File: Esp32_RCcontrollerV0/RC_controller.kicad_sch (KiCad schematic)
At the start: 15 parts, among them J1 Conn_01x03_Pin, J2 Conn_01x03_Pin, J3 Conn_01x02_Socket, J4 Conn_01x02_Socket, J5 5V_Signal, J6 5V_Signal, J7 INPUT POWER (12 - 24V), U1 XL1509-5.0, U2 NODEMCU-32S, U4 BOB-12009, U5 BOB-12009

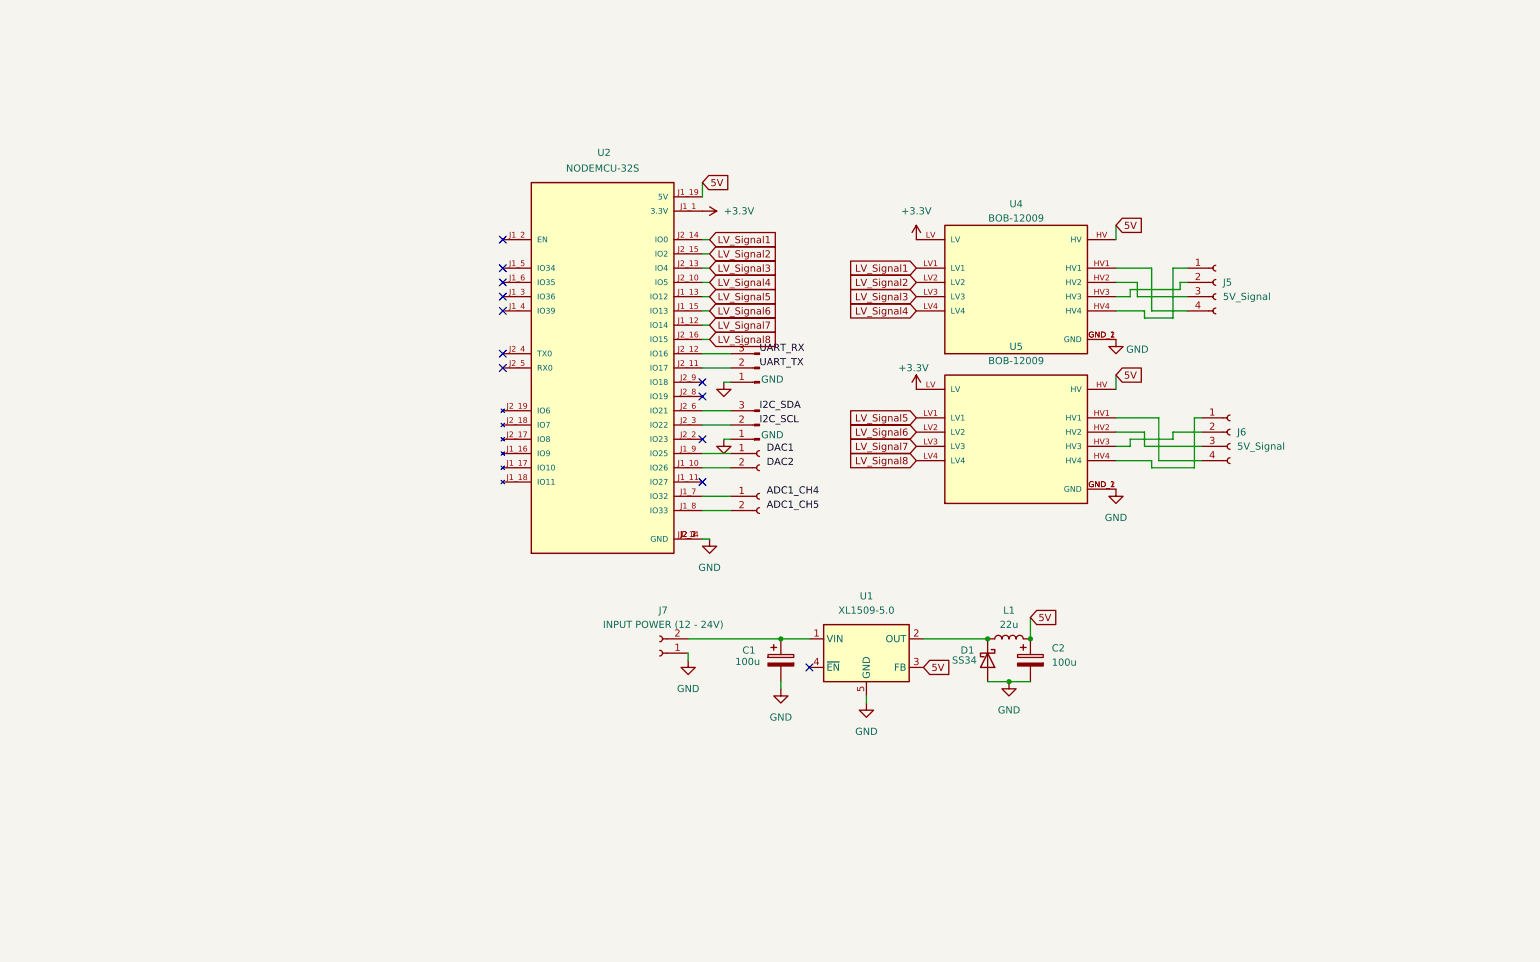
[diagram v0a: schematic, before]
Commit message: Core updates
Rework the board , Added Doc
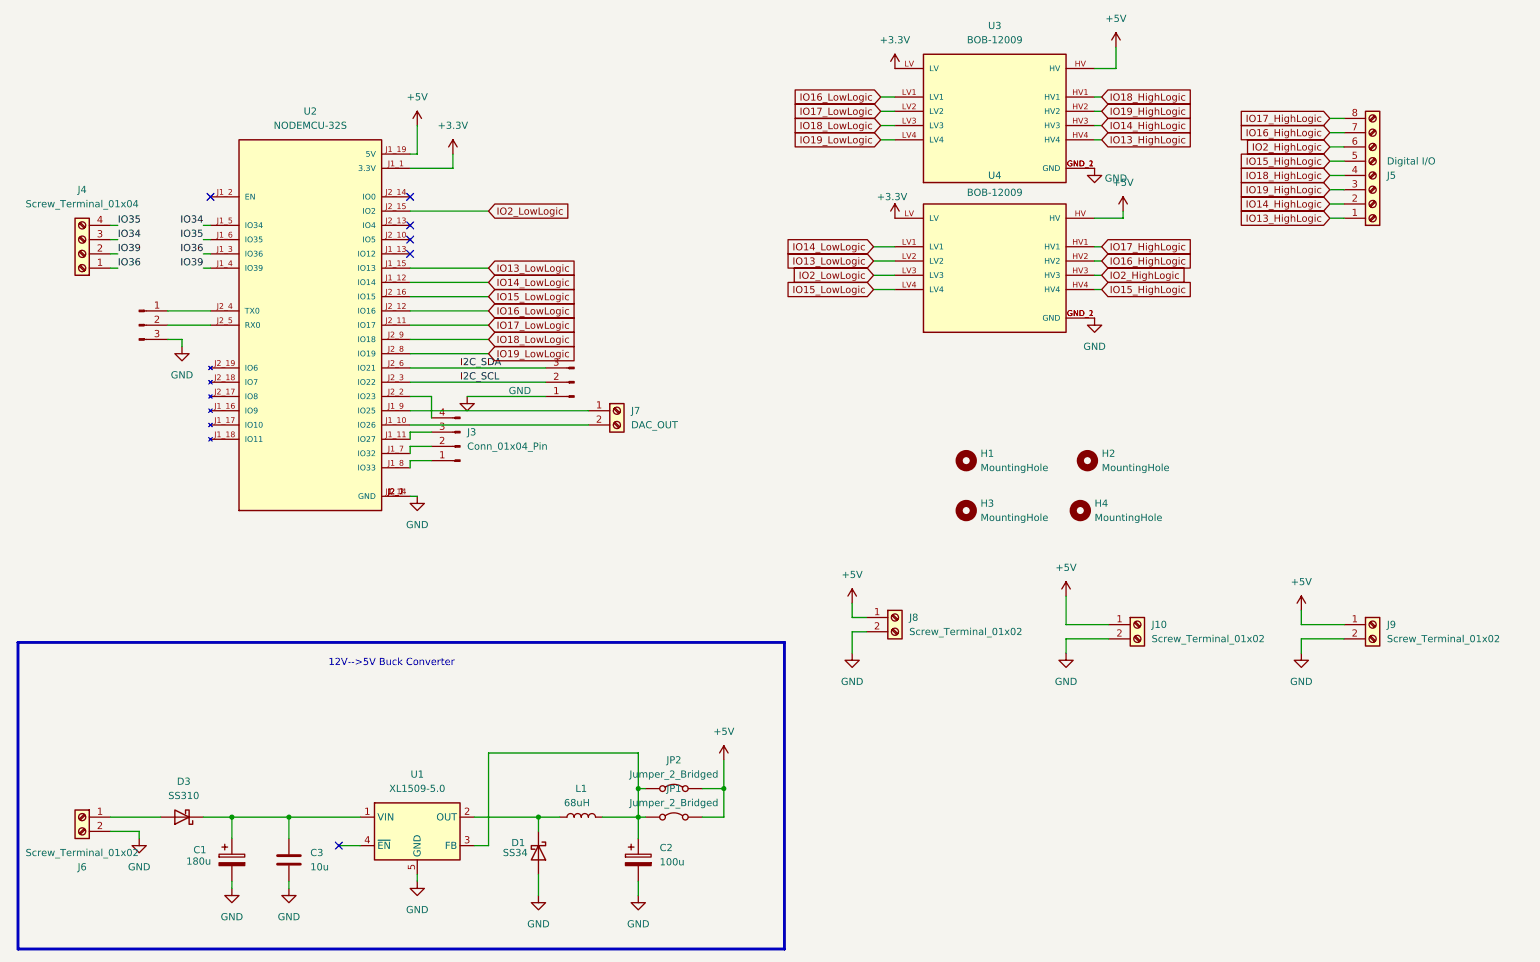
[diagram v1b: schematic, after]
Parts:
- removed J3, J4: Conn_01x02_Socket, TerminalBlock_Phoenix:TerminalBlock_Phoenix_PT-1,5-2-3.5-H_1x02_P3.50mm_Horizontal, symbol Connector:Conn_01x02_Socket
- removed J5, J6: 5V_Signal, TerminalBlock_Phoenix:TerminalBlock_Phoenix_PT-1,5-4-3.5-H_1x04_P3.50mm_Horizontal, symbol Connector:Conn_01x04_Socket
- removed J7: INPUT POWER (12 - 24V), TerminalBlock_Phoenix:TerminalBlock_Phoenix_MKDS-1,5-2-5.08_1x02_P5.08mm_Horizontal, symbol Connector:Conn_01x02_Socket
- removed U2: NODEMCU-32S, NODEMCU-32S:MODULE_NODEMCU-32S, symbol NODEMCU-32S:NODEMCU-32S
- removed U4, U5: BOB-12009, BOB-12009:CONV_BOB-12009, symbol BOB-12009:BOB-12009
- added C3: 10u, Capacitor_SMD:C_1206_3216Metric_Pad1.33x1.80mm_HandSolder, symbol Device:C
- added D3: SS310, Diode_SMD:D_SMA, symbol Diode:SS310
- added H1, H2, H3, H4: MountingHole, MountingHole:MountingHole_3.2mm_M3, symbol Mechanical:MountingHole
- added J10, J6, J8, J9: Screw_Terminal_01x02, TerminalBlock_Phoenix:TerminalBlock_Phoenix_PT-1,5-2-3.5-H_1x02_P3.50mm_Horizontal, symbol Connector:Screw_Terminal_01x02
- added J3: Conn_01x04_Pin, Connector_PinHeader_2.54mm:PinHeader_1x04_P2.54mm_Vertical, symbol Connector:Conn_01x04_Pin
- added J4: Screw_Terminal_01x04, TerminalBlock_Phoenix:TerminalBlock_Phoenix_PT-1,5-4-3.5-H_1x04_P3.50mm_Horizontal, symbol Connector:Screw_Terminal_01x04
- added J5: Digital I/O, TerminalBlock_Phoenix:TerminalBlock_Phoenix_PT-1,5-8-3.5-H_1x08_P3.50mm_Horizontal, symbol Connector:Screw_Terminal_01x08
- added J7: DAC_OUT, TerminalBlock_Phoenix:TerminalBlock_Phoenix_PT-1,5-2-3.5-H_1x02_P3.50mm_Horizontal, symbol Connector:Screw_Terminal_01x02
- added JP1, JP2: Jumper_2_Bridged, Connector_PinHeader_2.54mm:PinHeader_1x02_P2.54mm_Vertical, symbol Jumper:Jumper_2_Bridged
- added U2: NODEMCU-32S, LibMain:MODULE_NODEMCU-32S, symbol LibMain:NODEMCU-32S
- added U3, U4: BOB-12009, LibMain:CONV_BOB-12009, symbol LibMain:BOB-12009
- C1: value 100u -> 180u; footprint Capacitor_SMD:CP_Elec_10x10 -> Capacitor_THT:CP_Radial_D7.5mm_P2.50mm
- C2: footprint Capacitor_SMD:CP_Elec_6.3x5.8 -> Capacitor_THT:CP_Radial_D7.5mm_P2.50mm
- J1, J2: footprint Connector_JST:JST_EH_B3B-EH-A_1x03_P2.50mm_Vertical -> Connector_PinHeader_2.54mm:PinHeader_1x03_P2.54mm_Vertical
- L1: value 22u -> 68uH; footprint Inductor_SMD:L_APV_ANR5020 -> EasyEDA:IND-SMD_L7.1-W6.6_H5.0
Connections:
- net +3.3V: now also U2.J1_1 (3.3V), U3.LV, U4.LV
- net GND: now also J1.3 (Pin_3), C3.2, J10.2 (Pin_2), J6.2 (Pin_2), J8.2 (Pin_2), J9.2 (Pin_2), U2.J1_14 (GND), U2.J2_1 (GND), U2.J2_7 (GND), U3.GND_1 (GND), U3.GND_2 (GND), U4.GND_1 (GND), U4.GND_2 (GND); no longer J1.1 (Pin_1)
- net I2C_SCL: now also J2.2 (Pin_2), U2.J2_3 (IO22)
- net I2C_SDA: now also J2.3 (Pin_3), U2.J2_6 (IO21)
- net at C1.1, U1.1 (VIN): now also C3.1, D3.1 (K)
- net at J1.2 (Pin_2): now also U2.J2_5 (RX0)
- net 5V: no longer names the net of C2.1, L1.2, U1.3 (FB)
- net 5V: now also JP1.1 (A), JP2.1 (A)
- new net: D3.2 (A), J6.1 (Pin_1)
- new net: J3.1 (Pin_1), U2.J1_8 (IO33)
- new net: J3.2 (Pin_2), U2.J1_7 (IO32)
- new net: J3.3 (Pin_3), U2.J1_11 (IO27)
- new net: J3.4 (Pin_4), U2.J2_2 (IO23)
- new net: J7.2 (Pin_2), U2.J1_10 (IO26)
- new net: J7.1 (Pin_1), U2.J1_9 (IO25)
- new net: J1.1 (Pin_1), U2.J2_4 (TX0)
- new net +5V: J10.1 (Pin_1), J8.1 (Pin_1), J9.1 (Pin_1), JP1.2 (B), JP2.2 (B), U2.J1_19 (5V), U3.HV, U4.HV
- new net IO13_HighLogic: J5.1 (Pin_1), U3.HV4
- new net IO13_LowLogic: U2.J1_15 (IO13), U4.LV2
- new net IO14_HighLogic: J5.2 (Pin_2), U3.HV3
- new net IO14_LowLogic: U2.J1_12 (IO14), U4.LV1
- new net IO15_HighLogic: J5.5 (Pin_5), U4.HV4
- new net IO15_LowLogic: U2.J2_16 (IO15), U4.LV4
- new net IO16_HighLogic: J5.7 (Pin_7), U4.HV2
- new net IO16_LowLogic: U2.J2_12 (IO16), U3.LV1
- new net IO17_HighLogic: J5.8 (Pin_8), U4.HV1
- new net IO17_LowLogic: U2.J2_11 (IO17), U3.LV2
- new net IO18_HighLogic: J5.4 (Pin_4), U3.HV1
- new net IO18_LowLogic: U2.J2_9 (IO18), U3.LV3
- new net IO19_HighLogic: J5.3 (Pin_3), U3.HV2
- new net IO19_LowLogic: U2.J2_8 (IO19), U3.LV4
- new net IO2_HighLogic: J5.6 (Pin_6), U4.HV3
- new net IO2_LowLogic: U2.J2_15 (IO2), U4.LV3
- new net IO34: J4.3 (Pin_3), U2.J1_5 (IO34)
- new net IO35: J4.4 (Pin_4), U2.J1_6 (IO35)
- new net IO36: J4.1 (Pin_1), U2.J1_3 (IO36)
- new net IO39: J4.2 (Pin_2), U2.J1_4 (IO39)
- no-connect marks 12 -> 6
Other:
- note added: "12V-->5V Buck Converter"
- moved on the sheet: C1, C2, D1, L1, U1
